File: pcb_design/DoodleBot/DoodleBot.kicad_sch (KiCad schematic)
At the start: 20 parts

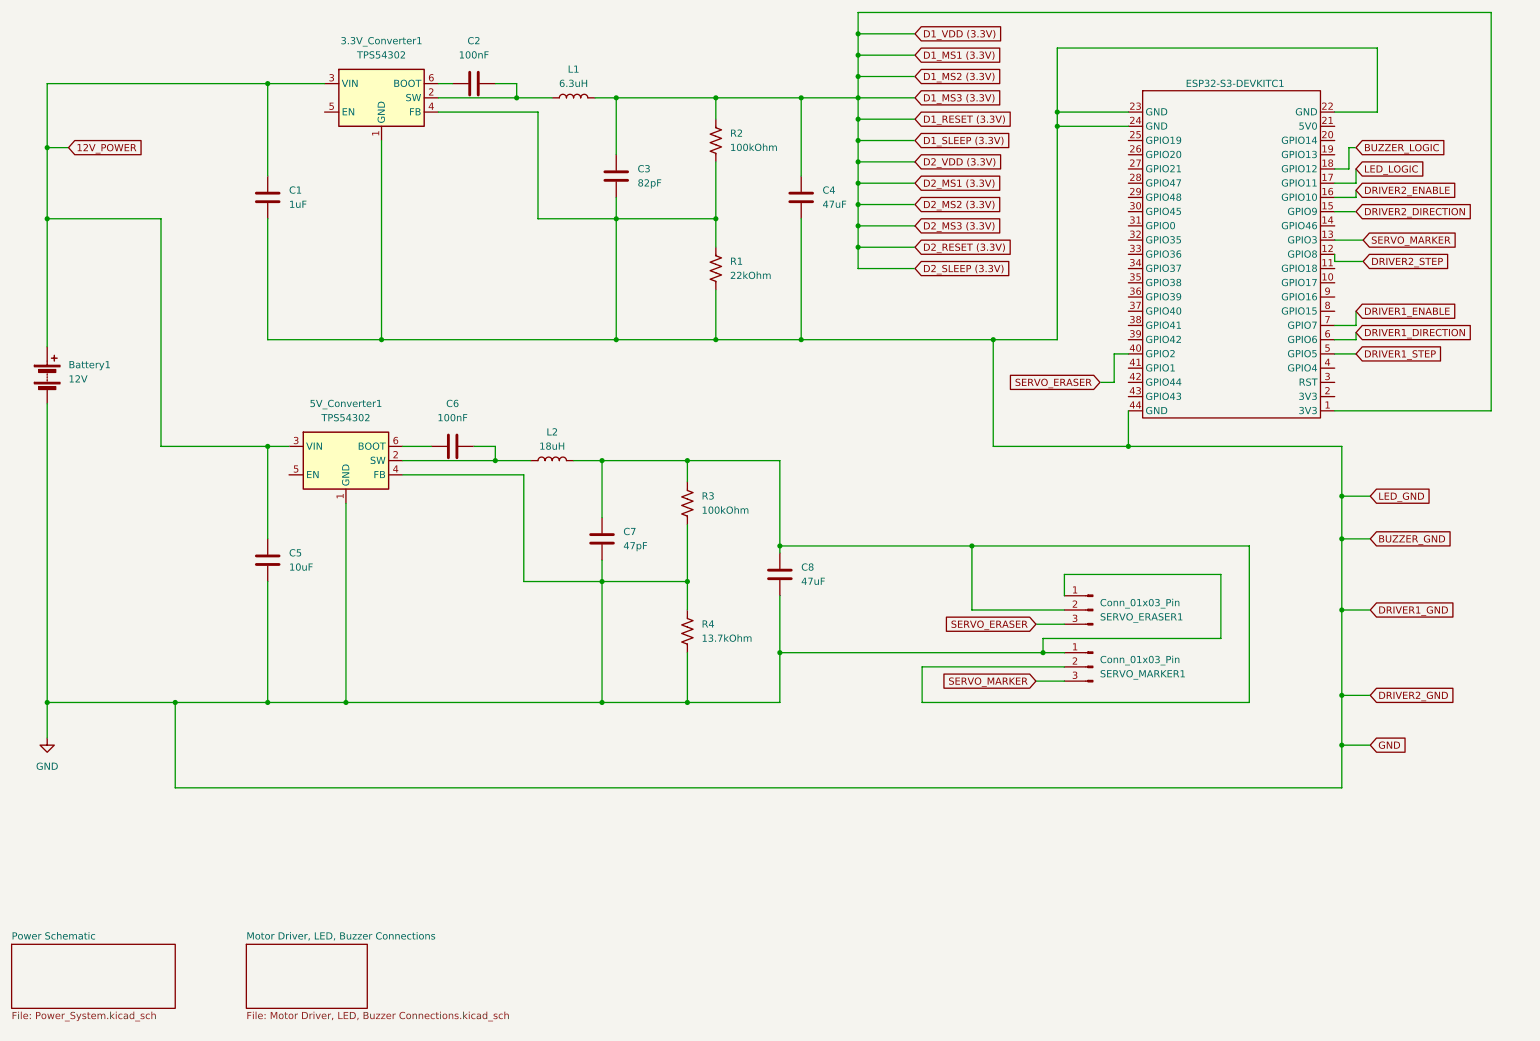
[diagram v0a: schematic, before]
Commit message: Connor's version
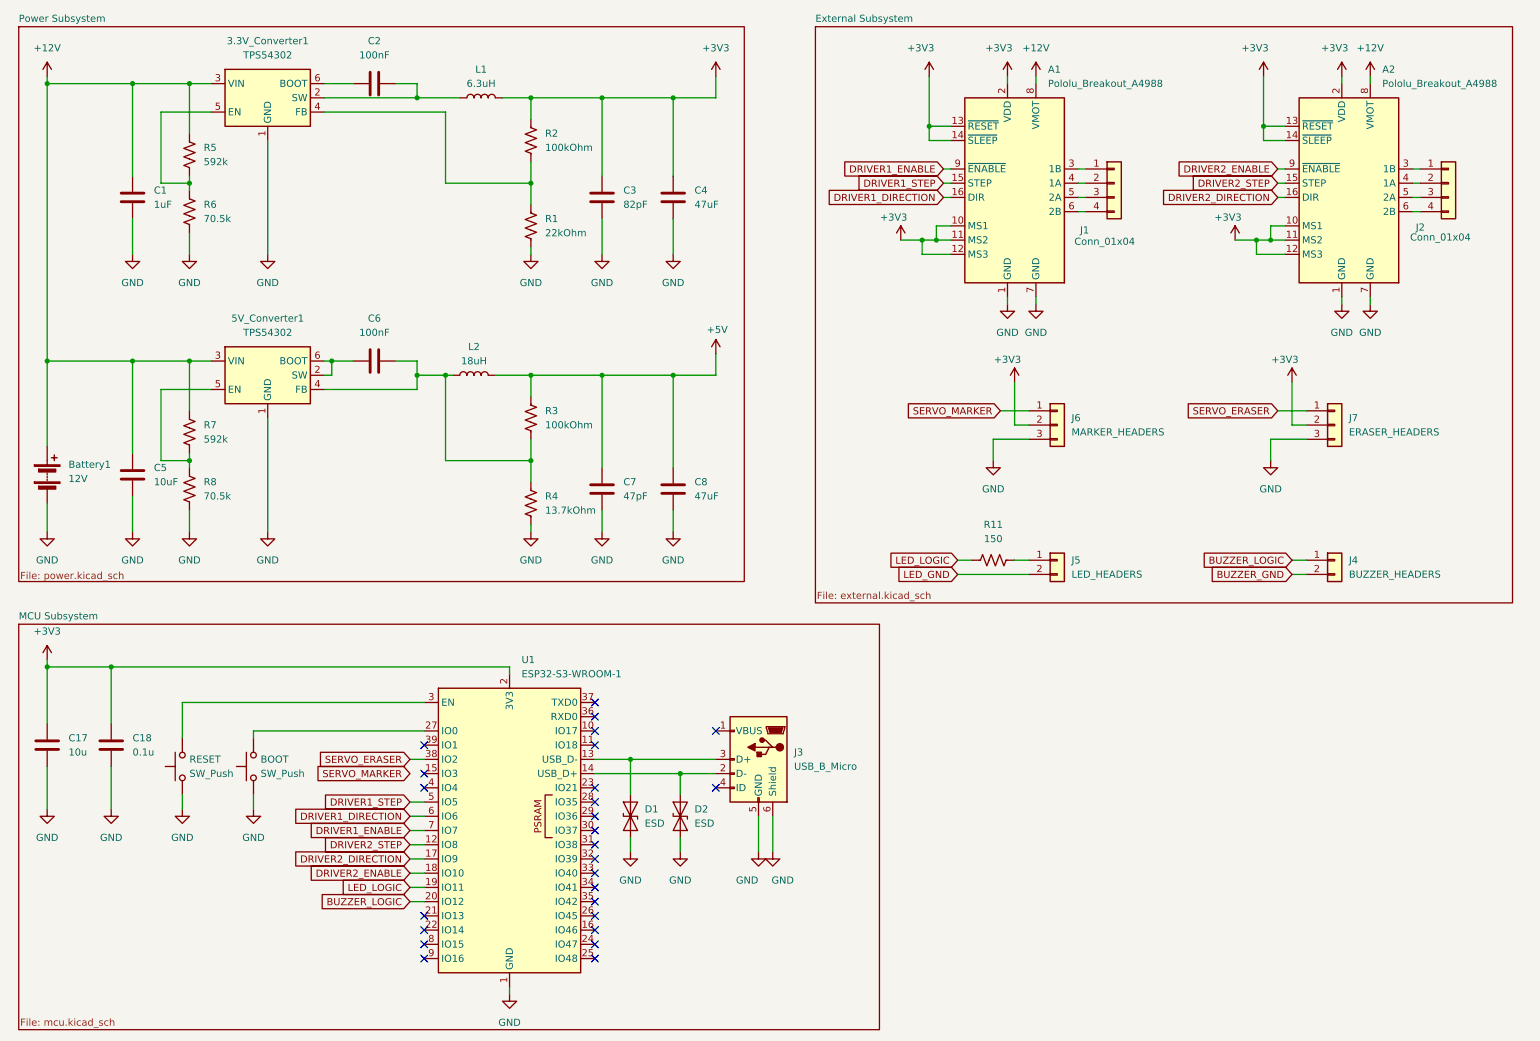
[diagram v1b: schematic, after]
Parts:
- removed ESP32-S3-DEVKITC1: ~, RF_Module:ESP32-S3-DEVKITC, symbol RF_Module:ESP32-S3-DEVKITC
- removed SERVO_ERASER1, SERVO_MARKER1: Conn_01x03_Pin, Connector_PinHeader_2.54mm:PinHeader_1x03_P2.54mm_Vertical, symbol Connector:Conn_01x03_Pin
- added A1, A2: Pololu_Breakout_A4988, Module:Pololu_Breakout-16_15.2x20.3mm, symbol Driver_Motor:Pololu_Breakout_A4988
- added BOOT, RESET: SW_Push, symbol Switch:SW_Push
- added C17: 10u, symbol Device:C
- added C18: 0.1u, symbol Device:C
- added D1, D2: ESD, Diode_SMD:Infineon_SG-WLL-2-3_0.58x0.28_P0.36mm, symbol Diode:ESD131-B1-W0201
- added J1, J2: Conn_01x04, symbol Connector_Generic:Conn_01x04
- added J3: USB_B_Micro, symbol Connector:USB_B_Micro
- added J4: BUZZER_HEADERS, symbol Connector_Generic:Conn_01x02
- added J5: LED_HEADERS, symbol Connector_Generic:Conn_01x02
- added J6: MARKER_HEADERS, symbol Connector_Generic:Conn_01x03
- added J7: ERASER_HEADERS, symbol Connector_Generic:Conn_01x03
- added R11: 150, Resistor_THT:R_Axial_DIN0204_L3.6mm_D1.6mm_P1.90mm_Vertical, symbol Device:R_US
- added R5, R7: 592k, symbol Device:R_US
- added R6, R8: 70.5k, symbol Device:R_US
- added U1: ESP32-S3-WROOM-1, RF_Module:ESP32-S3-WROOM-1, symbol RF_Module:ESP32-S3-WROOM-1
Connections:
- net BUZZER_LOGIC: now also J4.1 (Pin_1), U1.20 (IO12)
- net DRIVER1_DIRECTION: now also A1.16 (DIR), U1.6 (IO6)
- net DRIVER1_ENABLE: now also A1.9 (~{ENABLE}), U1.7 (IO7)
- net DRIVER1_STEP: now also A1.15 (STEP), U1.5 (IO5)
- net DRIVER2_DIRECTION: now also A2.16 (DIR), U1.17 (IO9)
- net DRIVER2_ENABLE: now also A2.9 (~{ENABLE}), U1.18 (IO10)
- net DRIVER2_STEP: now also A2.15 (STEP), U1.12 (IO8)
- net GND: now also A1.1 (GND), A1.7 (GND), A2.1 (GND), A2.7 (GND), BOOT.1, C17.2, C18.2, D1.1 (A1), D2.1 (A1), J3.5 (GND), J3.6 (Shield), J6.3 (Pin_3), J7.3 (Pin_3), R6.2, R8.2, RESET.1, U1.1 (GND), U1.40 (GND), U1.41 (GND); no longer 3.3V_Converter1.4 (FB), 5V_Converter1.4 (FB), R1.1, R2.2, R3.2, R4.1
- net LED_LOGIC: now also R11.1, U1.19 (IO11)
- net SERVO_ERASER: now also J7.1 (Pin_1), U1.38 (IO2)
- net SERVO_MARKER: now also J6.1 (Pin_1)
- net +5V: now reaches C7.2, C8.2, L2.2, R3.1
- net at C6.2, L2.1: now also 5V_Converter1.4 (FB), R3.2, R4.1; no longer 5V_Converter1.2 (SW)
- net at 5V_Converter1.5 (EN): now also R7.2, R8.1
- net at 5V_Converter1.6 (BOOT), C6.1: now also 5V_Converter1.2 (SW)
- net at 3.3V_Converter1.5 (EN): now also R5.2, R6.1
- net 12V_POWER renamed +12V
- net +12V: now also A1.8 (VMOT), A2.8 (VMOT), R5.1, R7.1
- net D1_MS1 (3.3V) renamed +3V3
- net +3V3: now also A1.10 (MS1), A1.11 (MS2), A1.12 (MS3), A1.13 (~{RESET}), A1.14 (~{SLEEP}), A1.2 (VDD), A2.10 (MS1), A2.11 (MS2), A2.12 (MS3), A2.13 (~{RESET}), A2.14 (~{SLEEP}), A2.2 (VDD), C17.1, C18.1, J6.2 (Pin_2), J7.2 (Pin_2), U1.2 (3V3)
- new net: 3.3V_Converter1.4 (FB), R1.1, R2.2
- new net: J5.1 (Pin_1), R11.2
- new net: RESET.2, U1.3 (EN)
- new net: A2.3 (1B), J2.1 (Pin_1)
- new net: A2.4 (1A), J2.2 (Pin_2)
- new net: A2.5 (2A), J2.3 (Pin_3)
- new net: A2.6 (2B), J2.4 (Pin_4)
- new net: D1.2 (A2), J3.3 (D+), U1.13 (USB_D-)
- new net: A1.3 (1B), J1.1 (Pin_1)
- new net: A1.4 (1A), J1.2 (Pin_2)
- new net: A1.5 (2A), J1.3 (Pin_3)
- new net: A1.6 (2B), J1.4 (Pin_4)
- new net: D2.2 (A2), J3.2 (D-), U1.14 (USB_D+)
- new net: BOOT.2, U1.27 (IO0)
- new net BUZZER_GND: J4.2 (Pin_2)
- new net LED_GND: J5.2 (Pin_2)
- no-connect marks 0 -> 26
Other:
- removed sheet Motor Driver, LED, Buzzer Connections
- removed sheet Power Schematic
- added sheet External Subsystem (external.kicad_sch)
- added sheet MCU Subsystem (mcu.kicad_sch)
- added sheet Power Subsystem (power.kicad_sch)
- title: (none) -> DoodleBot Full Schematic
- moved on the sheet: 3.3V_Converter1, 5V_Converter1, Battery1, C1, C2, C3, C4, C5, C6, C7, C8, L1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
